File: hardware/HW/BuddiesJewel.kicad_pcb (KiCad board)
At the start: 2 copper layers, 24 parts, among them CON1 AVR-ISP6, CON2 ANTENNE, IC1 ATTINY25-P, P1 ALIM, U1 PT, U2 PT, U3 PT, U4 PT, U5 RF430CL330H

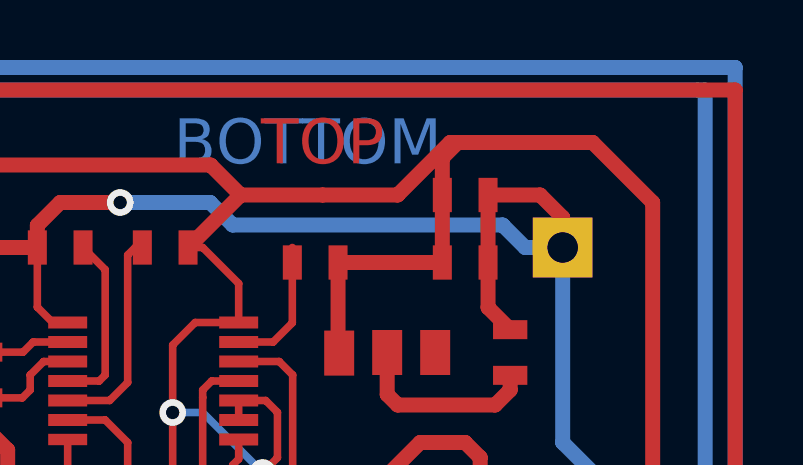
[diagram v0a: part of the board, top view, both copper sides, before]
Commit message: (minor) modif on pcb
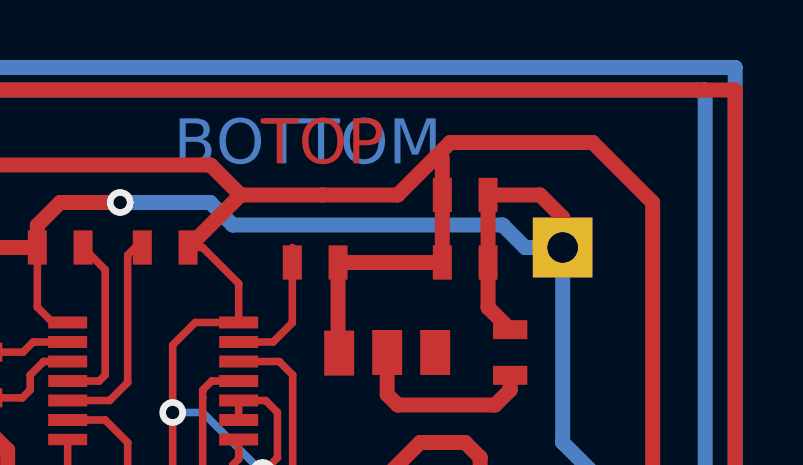
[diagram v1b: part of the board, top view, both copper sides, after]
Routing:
- net GND: track 111.2 -> 110.4 mm
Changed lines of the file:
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@@
   (general
     (links 53)
-    (no_connects 0)
-    (area 48.861 21.336 91.406001 59.275)
+    (no_connects 1)
+    (area 0 0 0 0)
     (thickness 1.6)
     (drawings 12)
-    (tracks 218)
+    (tracks 217)
     (zones 0)
     (modules 24)
@@
     (visible_elements 7FFFFFDF)
     (pcbplotparams
-      (layerselection 3178497)
+      (layerselection 16809985)
       (usegerberextensions true)
       (excludeedgelayer true)
@@
       (outputformat 1)
       (mirror false)
-      (drillshape 1)
+      (drillshape 0)
       (scaleselection 1)
-      (outputdirectory svg))
+      (outputdirectory percage))
   )
   (net 0 "")
@@
   (segment (start 71.25 30) (end 68.75 30) (width 0.5) (layer Dessus.Cu) (net 9))
   (segment (start 73 28.25) (end 71.25 30) (width 0.5) (layer Dessus.Cu) (net 9))
-  (segment (start 73.25 28.25) (end 72.738 28.762) (width 0.5) (layer Dessus.Cu) (net 9))
   (segment (start 77.75 28.25) (end 73.25 28.25) (width 0.5) (layer Dessus.Cu) (net 9))
   (segment (start 79.75 30.25) (end 77.75 28.25) (width 0.5) (layer Dessus.Cu) (net 9))
